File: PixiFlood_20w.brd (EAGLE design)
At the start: 43 x 46 mm, 35 parts, among them IC1 WS2811-SOP8, IC3 L78LXXCU/BU, T1 BC846, T2 BC846, T3 BC846, U1 PT4115B89E, U2 PT4115B89E, U3 PT4115B89E, X2 22-23-2041

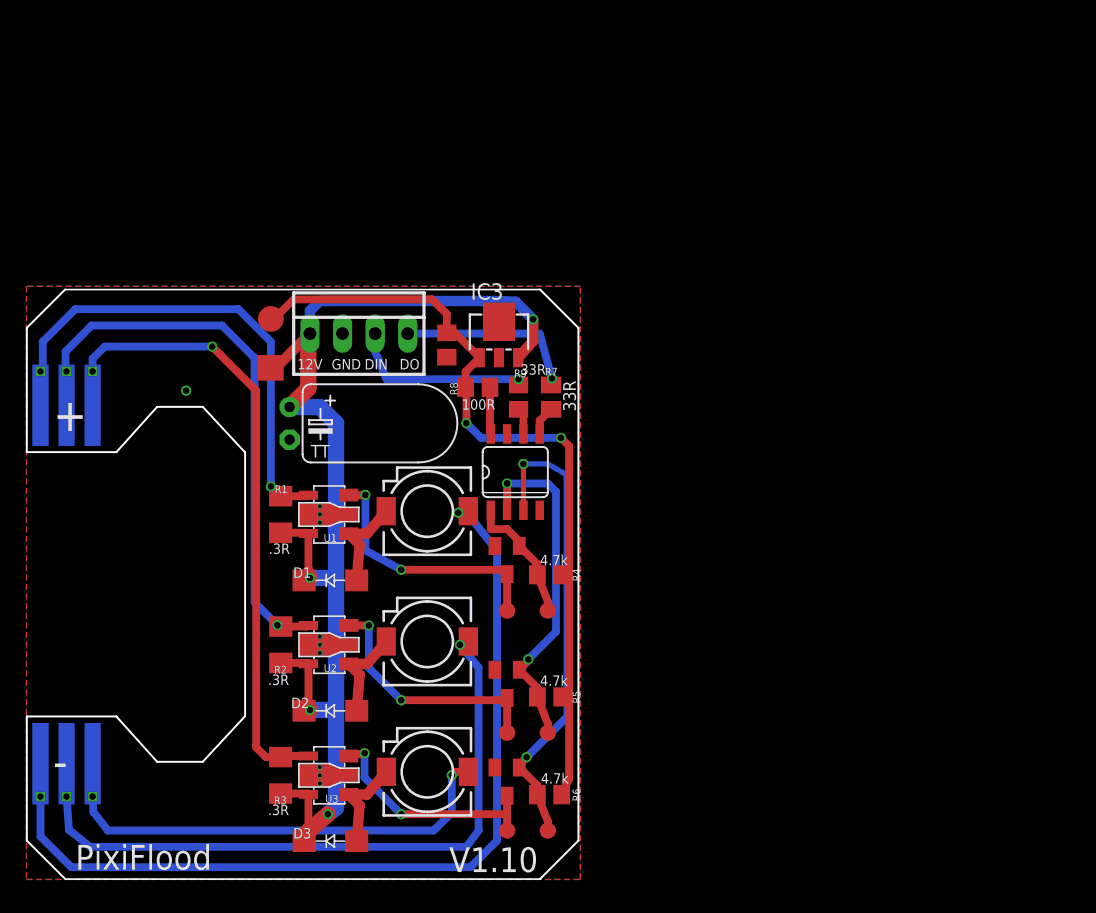
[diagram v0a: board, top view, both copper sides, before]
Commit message: added 20w board
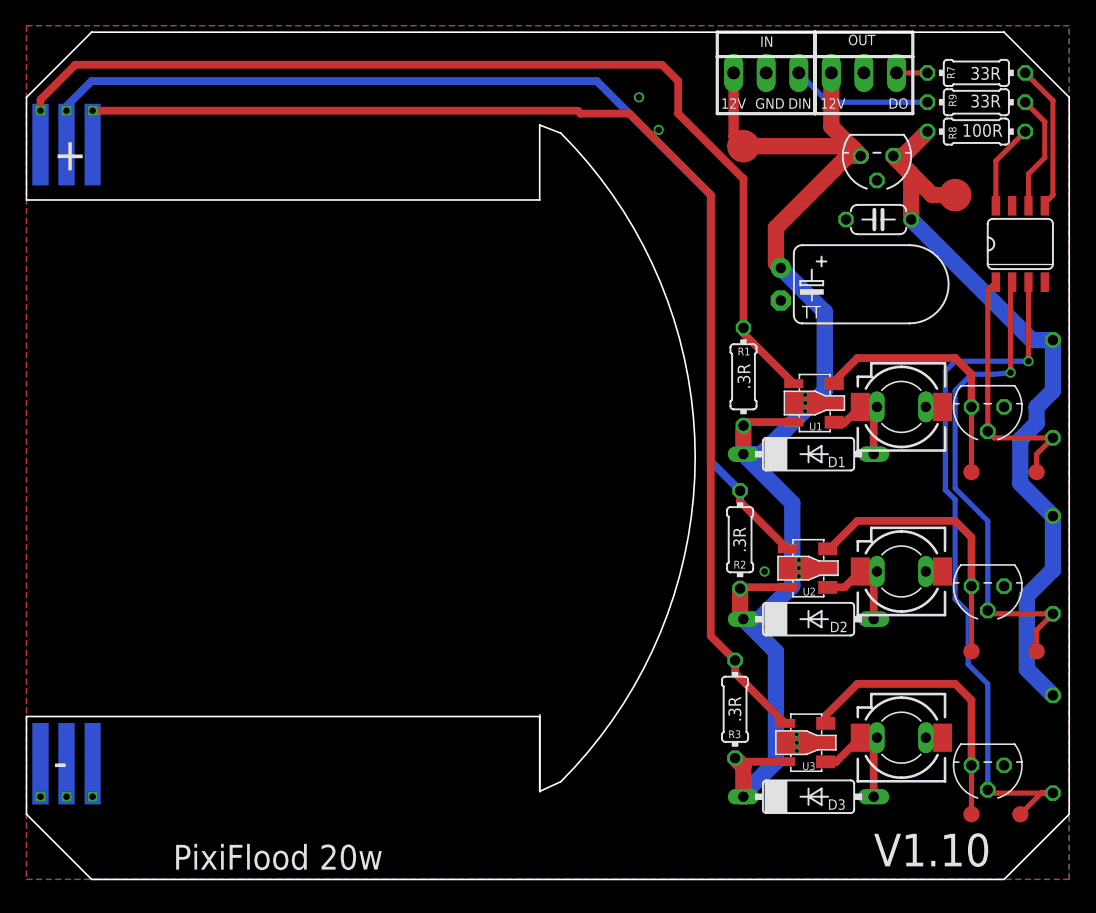
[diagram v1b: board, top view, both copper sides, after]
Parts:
- removed IC3: L78LXXCU/BU, regulators:SOT89
- added IC2: 78L05Z, linear:TO92
- added X1: 22-23-2031, MyLibrary:22-23-2031
- B1: value LED-BOARDV4 -> LED-BOARD20W-30W; device special:LED_BOARD-V4 -> special:LED-BOARD-LRG
- C2: device rcl:C0805 -> rcl:C050-024X044
- D1, D2, D3: device diode:SMA-DO214AC -> diode:DO07
- L1, L2, L3: value SLF7045 -> 82114RPTH_SMD; device inductors:SLF7045 -> inductors:INDUCTOR
- R1, R2, R3: device resistor:R1206 -> resistor:0204/7
- R4, R5, R6: device resistor:R0805 -> resistor:0204/7
- R7: device rcl:M0805 -> rcl:0204/7
- R8, R9: device rcl:R0805 -> rcl:0204/7
- T1, T2, T3: value BC846 -> 2N3904; device transistor:SOT23 -> transistor:TO92
- TP1: value PTR1TP20SQ -> PTR1B2,54; device testpad:TP20SQ -> testpad:B2,54
- TP2: value PTR1TP20R -> PTR1B2,54; device testpad:TP20R -> testpad:B2,54
- X2: value 22-23-2041 -> 22-23-2031; device connectors:22-23-2041 -> MyLibrary:22-23-2031
- moved TP2 54.2 mm to (72.4, 53.3)
- moved R8 43.7 mm to (74.0, 58.3)
- moved IC1 43.2 mm to (77.5, 49.5)
- moved R9 42.4 mm to (74.0, 60.6), turned to 0 degrees
- moved R4 41.8 mm to (80.0, 38.2), flipped to the bottom, turned to 270 degrees
- moved R7 41.7 mm to (74.0, 62.9), turned to 0 degrees
- moved TP1 40.7 mm to (55.9, 57.1), turned to 0 degrees
- moved R5 40.6 mm to (80.0, 24.5), flipped to the bottom, turned to 270 degrees
- moved C1 39.8 mm to (58.8, 46.4)
- moved TP3 39.6 mm to (78.7, 31.8)
- moved R6 39.4 mm to (80.0, 10.5), flipped to the bottom, turned to 270 degrees
- moved T1 39.3 mm to (74.9, 36.8)
- moved U1 38.8 mm to (61.5, 37.1)
- moved TP5 38.6 mm to (78.7, 17.8)
- moved D1 38.5 mm to (61.0, 33.1), turned to 0 degrees
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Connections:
- net +12V: now also D1.C, D2.C, D3.C, IC2.3, X1.1; no longer D1.K, D2.K, D3.K, IC3.3
- net +5V: now also IC2.1; no longer IC3.1
- net BLUE: now also T3.1; no longer T3.3
- net GND: now also IC2.2, T1.3, T2.3, T3.3, X1.2; no longer IC3.4, T1.2, T2.2, T3.2
- net GREEN: now also T2.1; no longer T2.3
- net N$1: now also L1.1@A
- net N$10: now also L3.2@A
- net N$15: now also T3.2; no longer T3.1
- net N$18: now also T2.2; no longer T2.1
- net N$2: now also L3.1@A
- net N$20: now also T1.2; no longer T1.1
- net N$3: now also L1.2@A
- net N$4: now also X1.3; no longer X2.4
- net N$5: now also L2.1@A
- net N$9: now also L2.2@A
- net RED: now also T1.1; no longer T1.3
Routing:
- net N$3: track 70.9 -> 0.00 mm, vias 1 -> 0
- net N$9: track 54.0 -> 0.00 mm, vias 1 -> 0
- net BOUT: track 50.8 -> 97.1 mm, vias 1 -> 0
- net GOUT: track 47.6 -> 87.8 mm, vias 1 -> 0
- net ROUT: track 42.1 -> 82.2 mm, vias 1 -> 0
- net N$10: track 37.3 -> 0.00 mm, vias 1 -> 0
- net N$15: track 37.3 -> 55.4 mm, vias 2 -> 1
- net N$4: track 14.4 -> 2.41 mm, vias 1 -> 0
- net N$18: track 27.0 -> 38.8 mm, vias 2 -> 1
- net +12V: track 95.2 -> 106.4 mm, vias 4 -> 0
- net N$20: track 10.2 -> 20.4 mm
- net N$7: track 2.29 -> 11.5 mm
- net N$8: track 2.08 -> 9.23 mm
- net BLUE: track 18.2 -> 22.4 mm, vias 2 -> 0
- net N$6: track 14.5 -> 11.0 mm, vias 1 -> 0
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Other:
- board size 43 x 46 mm -> 81.3 x 66 mm
- board text added: "IN"
- board text added: "OUT"
- board text added: "PixiFlood 20w"
- board text removed: "PixiFlood"
